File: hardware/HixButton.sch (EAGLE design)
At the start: 16 parts, among them J1 FTDI, J3 XH2P

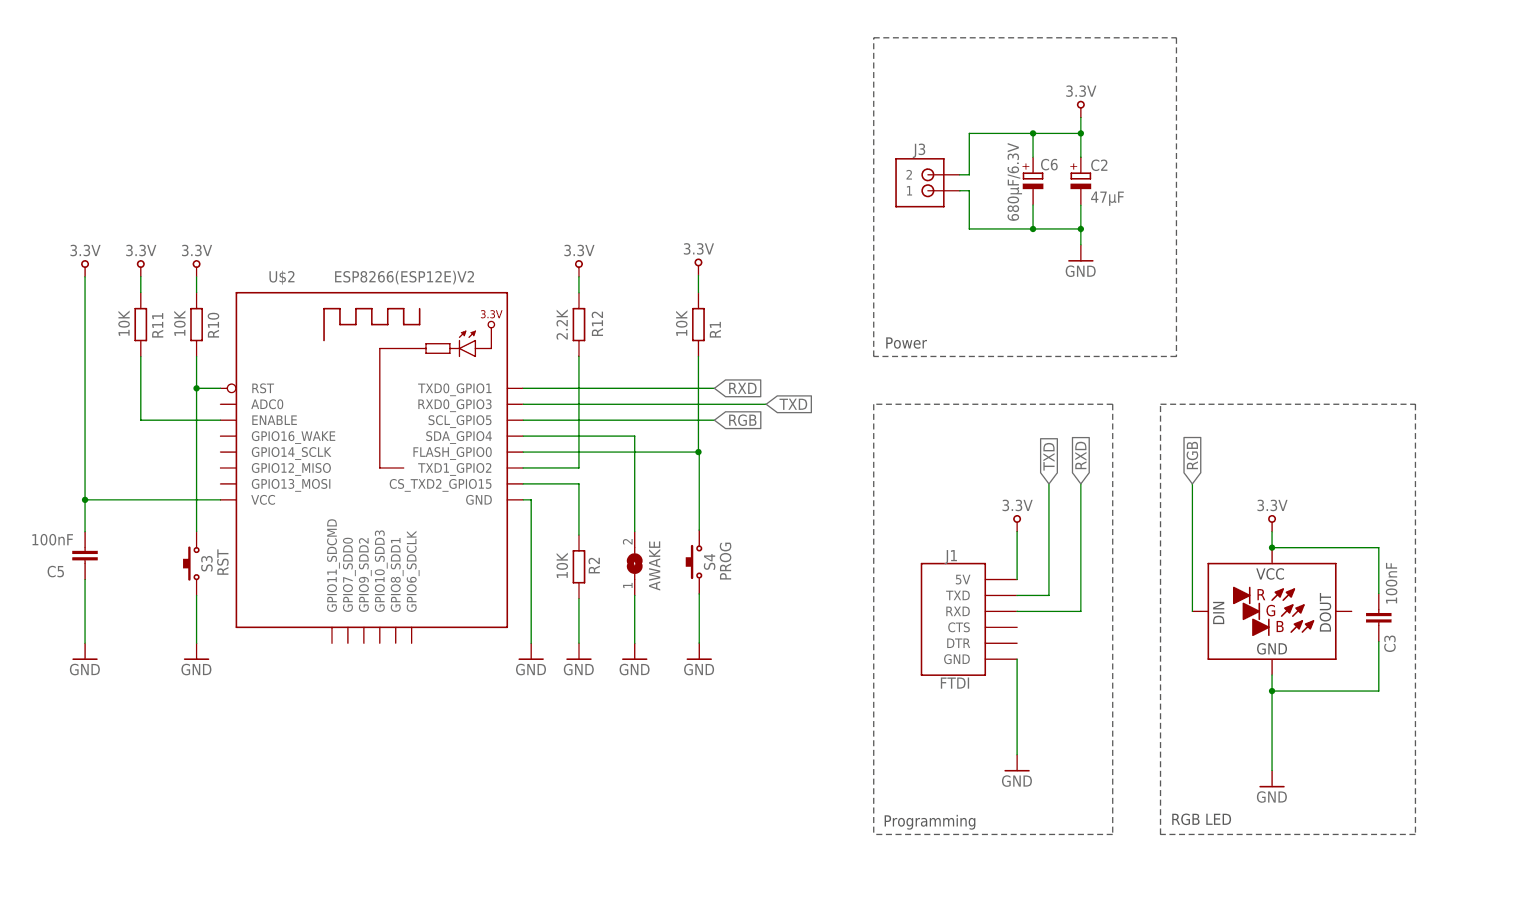
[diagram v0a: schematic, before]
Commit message: hardware update
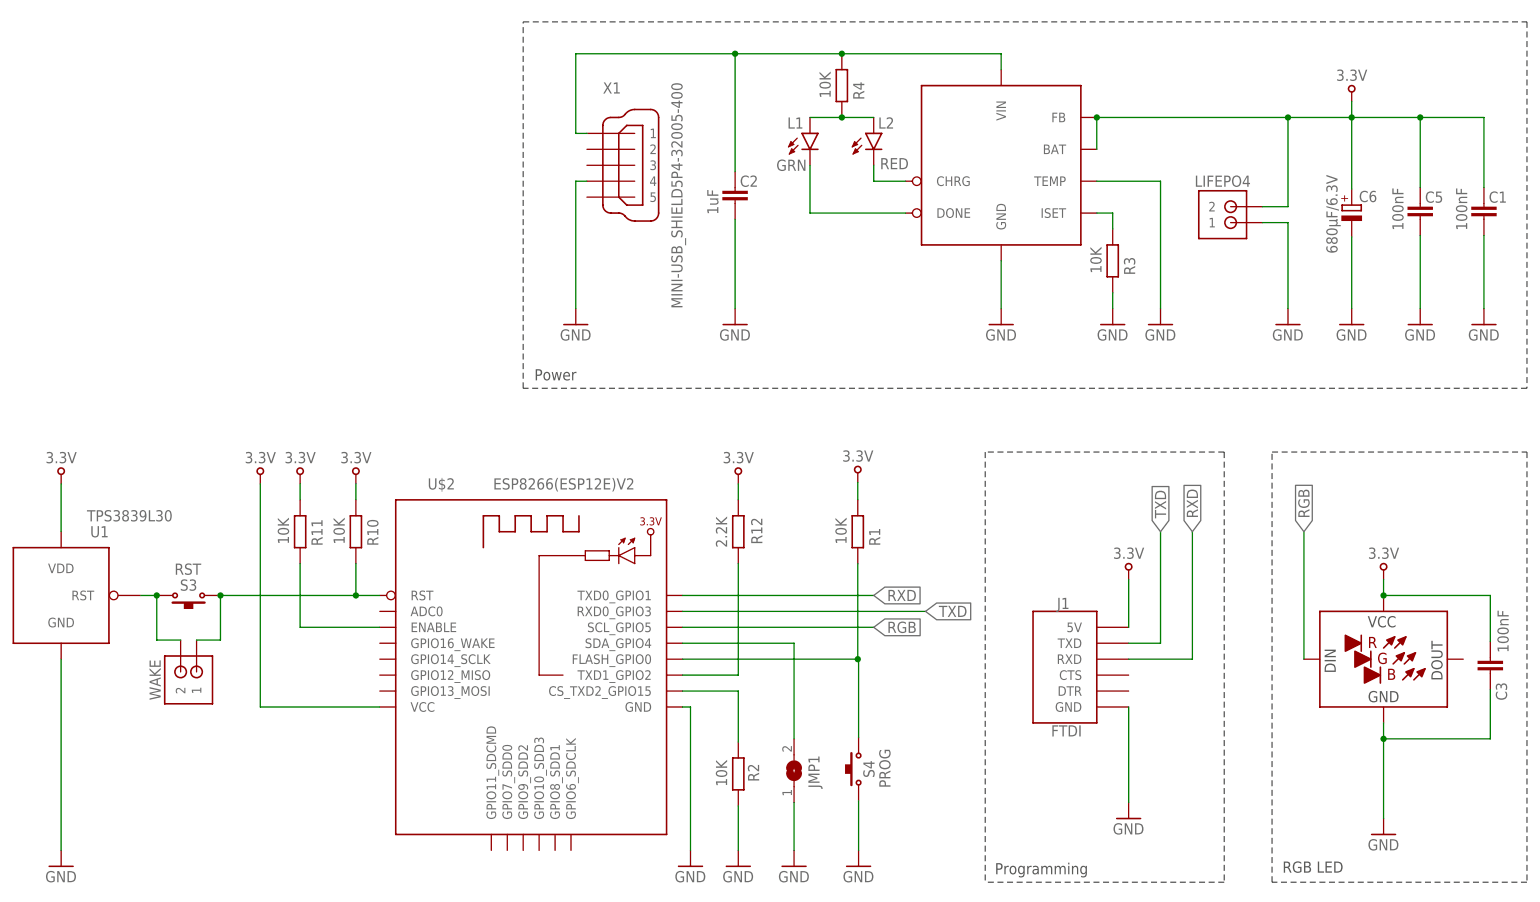
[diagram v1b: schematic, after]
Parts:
- removed AWAKE: (no value), jumper:SJ
- removed J3: XH2P, 0_HixField:XH2P
- added C1: 100nF, rcl:C-EUC1206
- added JMP1: (no value), jumper:SJ
- added L1: GRN, led:LEDCHIPLED_1206
- added L2: RED, led:LEDCHIPLED_1206
- added LIFEPO4, WAKE: XH2P, 0_HixField:XH2P
- added R3, R4: 10K, rcl:R-EU_R1206
- added U$1: CN3058E, 0_HixField:CN3058E
- added U1: TPS3839L30, 0_HixField:TPS3839
- added X1: MINI-USB_SHIELD5P4-32005-400, con-cypressindustries:MINI-USB_SHIELD5P4-32005-400
- C2: value 47μF -> 1uF; device rcl:CPOL-EUSMCA -> rcl:C-EUC1206
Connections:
- removed net N$7: R10.1, S3.1, U$2.RST
- new net N$10: C2.1, R4.2, U$1.VIN, X1G$1.1
- new net N$11: L1.A, L2.A, R4.1
- new net N$12: L2.C, U$1.CHRG
- new net N$13: L1.C, U$1.DONE
- new net N$5: R10.1, S3.2, U$2.RST, WAKE.1
- new net N$6: R3.2, U$1.ISET
- new net N$9: S3.1, U1.RST, WAKE.2
- net 3.3V: now also C1.1, LIFEPO4.2, U$1.BAT, U$1.FB, U1.VDD; no longer C2.+, J3.2
- net GND: now also C1.2, C2.2, JMP1.1, LIFEPO4.1, R3.1, U$1.GND, U$1.TEMP, U1.GND, X1G$1.4; no longer AWAKE.1, C2.-, J3.1, S3.2
- net N$4: now also JMP1.2; no longer AWAKE.2
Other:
- moved on the sheet: C3, C5, C6, J1, R1, R10, R11, R12, R2, S3, S4, U$2
